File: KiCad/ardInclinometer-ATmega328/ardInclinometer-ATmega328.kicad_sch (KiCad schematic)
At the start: 26 parts, among them SW1 Lock X, SW2 Lock Y, SW3 Lock Z, SW4 Lock all, SW5 SW_Push, U1 GY-521_MPU-6050, U2 SSD1306_I2C_display

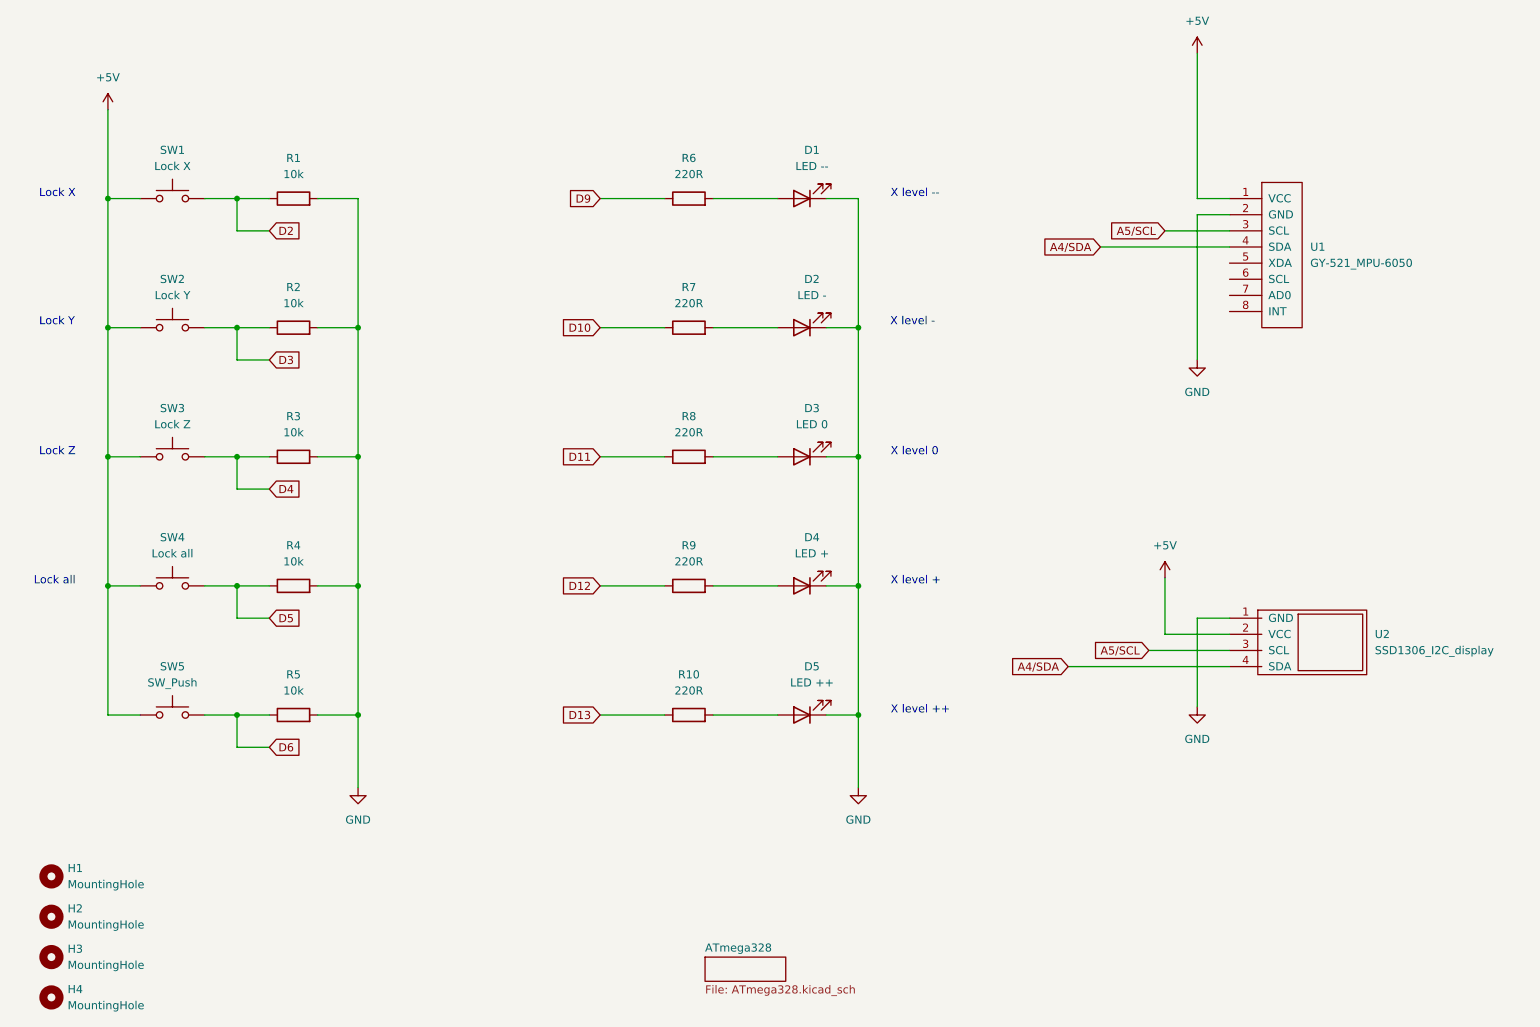
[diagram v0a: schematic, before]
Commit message: kicad corrections and dev
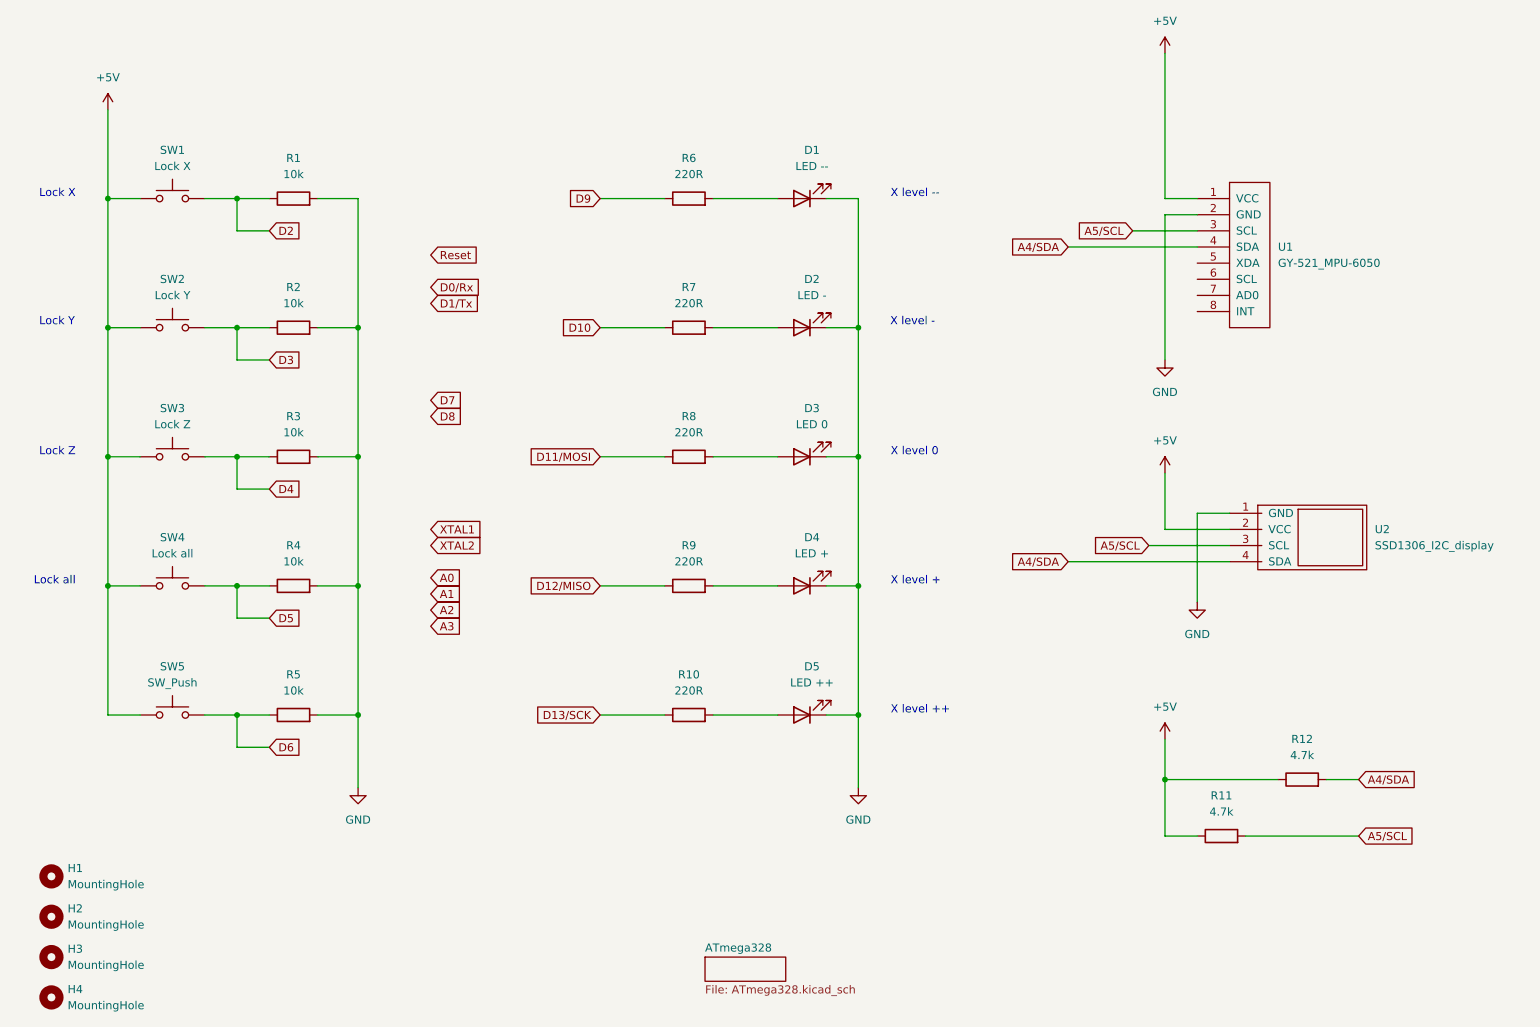
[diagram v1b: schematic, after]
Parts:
- added R11, R12: 4.7k, My_Misc:R_Axial_DIN0207_L6.3mm_D2.5mm_P10.16mm_Horizontal_large, symbol Device:R
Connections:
- net +5V: now also R11.1, R12.1
- net A4/SDA: now also R12.2
- net A5/SCL: now also R11.2
- net D11 renamed D11/MOSI
- net D12 renamed D12/MISO
- net D13 renamed D13/SCK
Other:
- moved on the sheet: U1, U2
